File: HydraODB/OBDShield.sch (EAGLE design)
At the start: 10 parts, among them J1 HYDRABUS_SHIELD_CON_HEADER_2X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, J2 HYDRABUS_SHIELD_CON_HEADER_2X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, J3 HYDRABUS_SHIELD_CON_HEADER_2X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, U1 SN65HVD233DG4, U2 SN65HVD233DG4

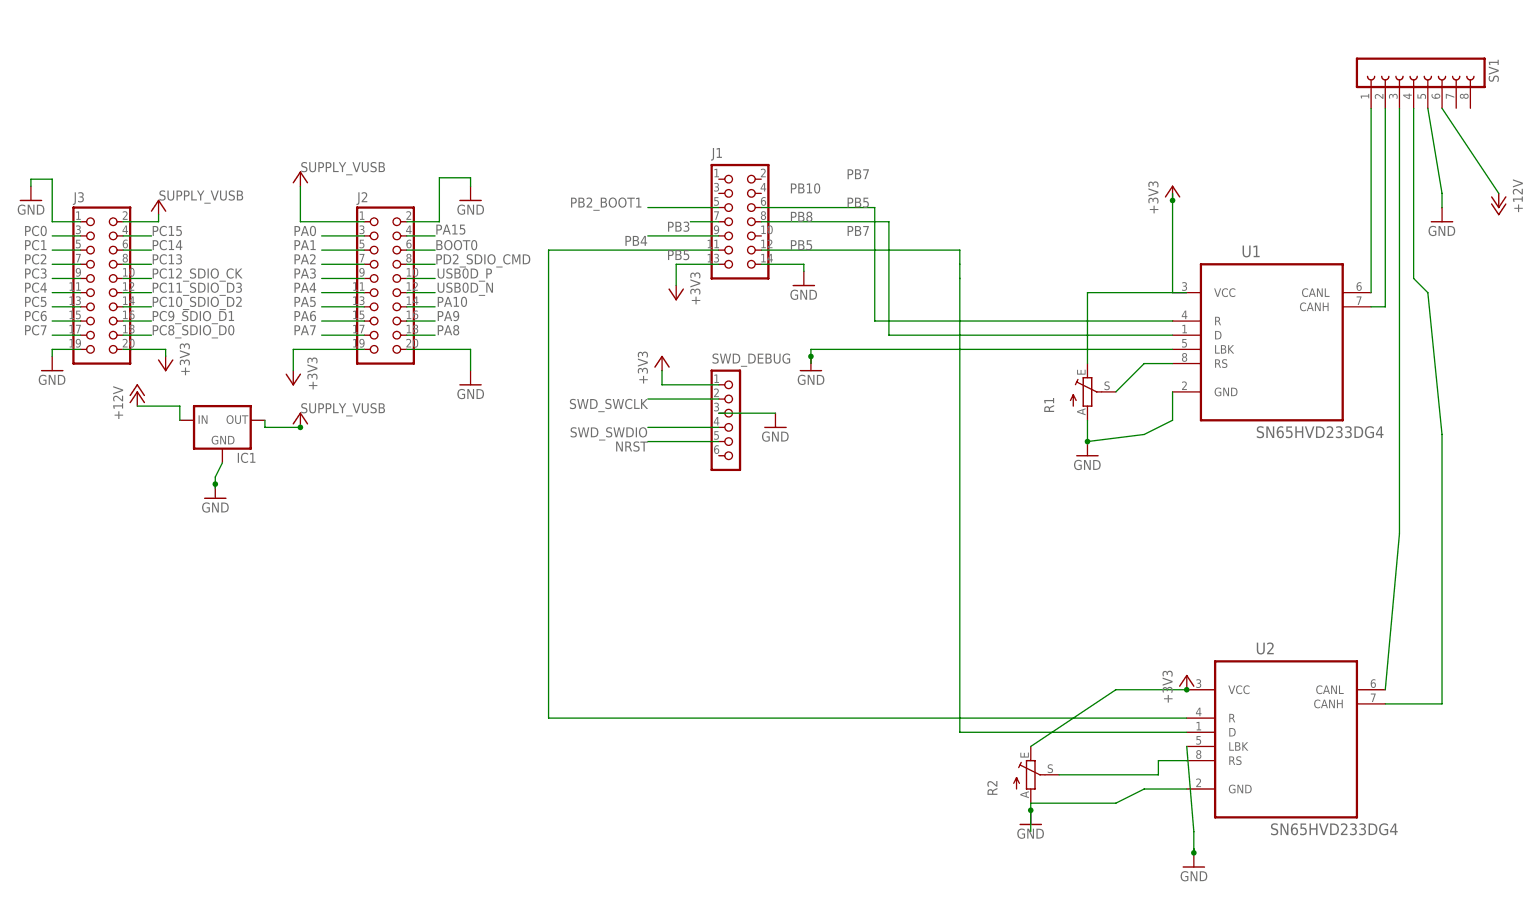
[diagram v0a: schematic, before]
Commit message: Mistake :-D
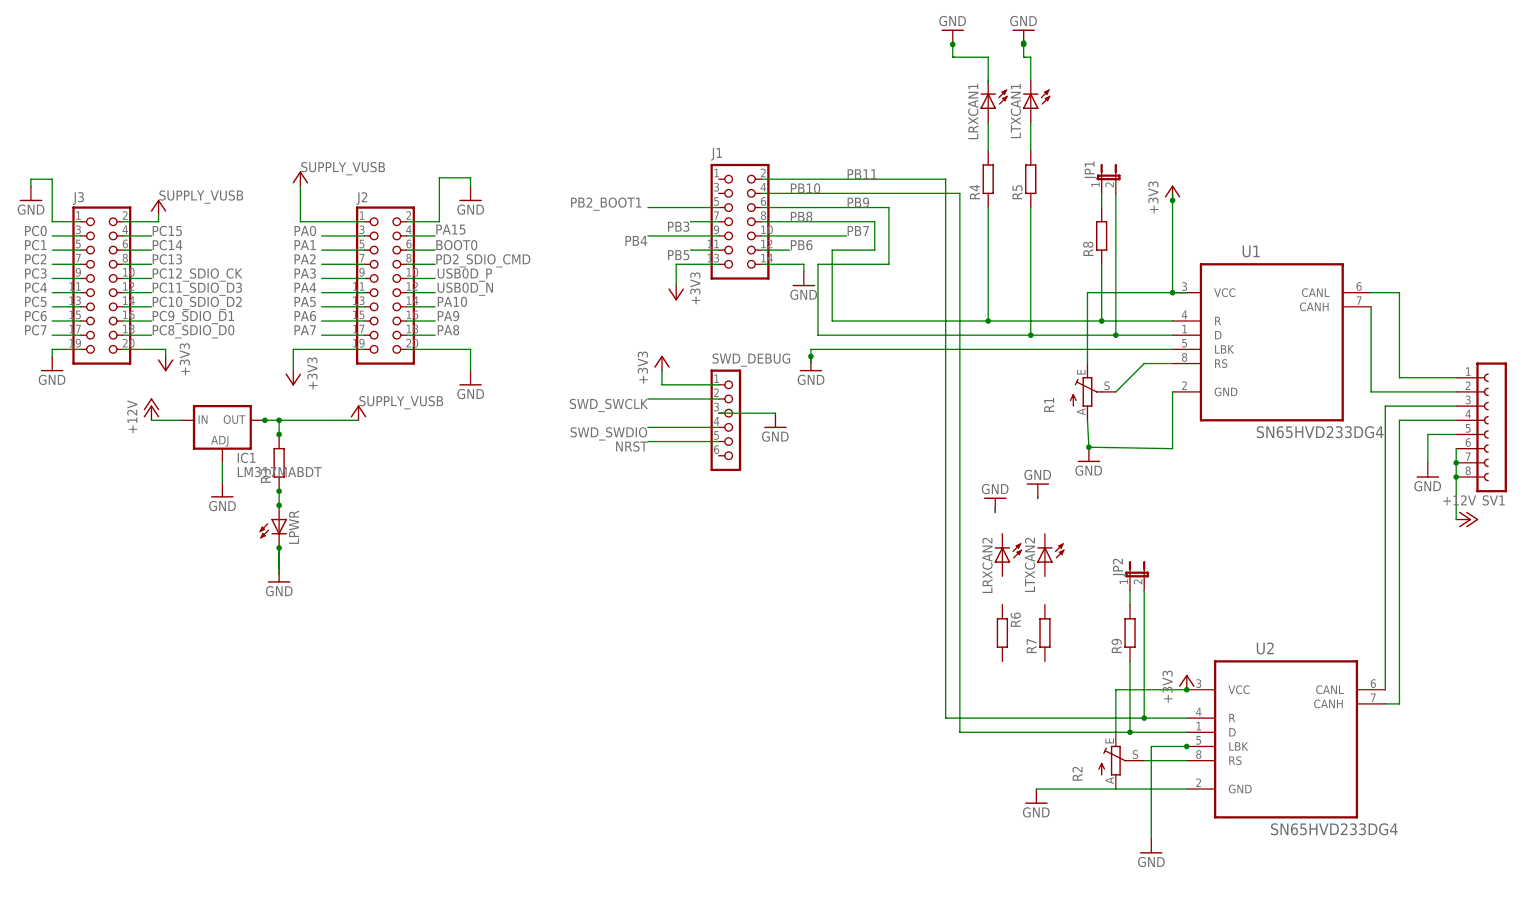
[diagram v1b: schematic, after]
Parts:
- added JP1, JP2: (no value), jumper:JP1E
- added LPWR, LRXCAN1, LRXCAN2, LTXCAN1, LTXCAN2: (no value), led:LEDCHIPLED_0603
- added R3, R4, R5, R6, R7, R8, R9: (no value), resistor:R-EU_R0603
- IC1: value (none) -> LM317MABDT; device v-reg:78XXS -> v-reg:LM317MABDT
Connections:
- new net N$13: LTXCAN1.A, R5.2
- new net N$14: LPWR.A, R3.1
- new net N$15: R3.2
- new net N$16: JP2.1, R9.2
- new net N$19: JP1.1, R8.2
- new net N$7: LRXCAN1.A, R4.2
- new net PB11: J1.4, R9.1, U2.D
- new net PB6: J1.12
- new net PB9: J1.2, JP2.2, U2.R
- net +12V: now also SV1.7, SV1.8
- net GND: now also IC1.ADJ, LPWR.C, LTXCAN1.C; no longer IC1.GND
- net PB10: now also J1.6, JP1.2, R5.1; no longer J1.8
- net PB5: no longer U2.R
- net PB7: now also J1.10; no longer J1.12, U2.D
- net PB8: now also J1.8, R4.1, R8.1; no longer J1.6
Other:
- moved on the sheet: R2, SV1
